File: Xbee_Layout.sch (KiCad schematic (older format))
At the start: 28 parts

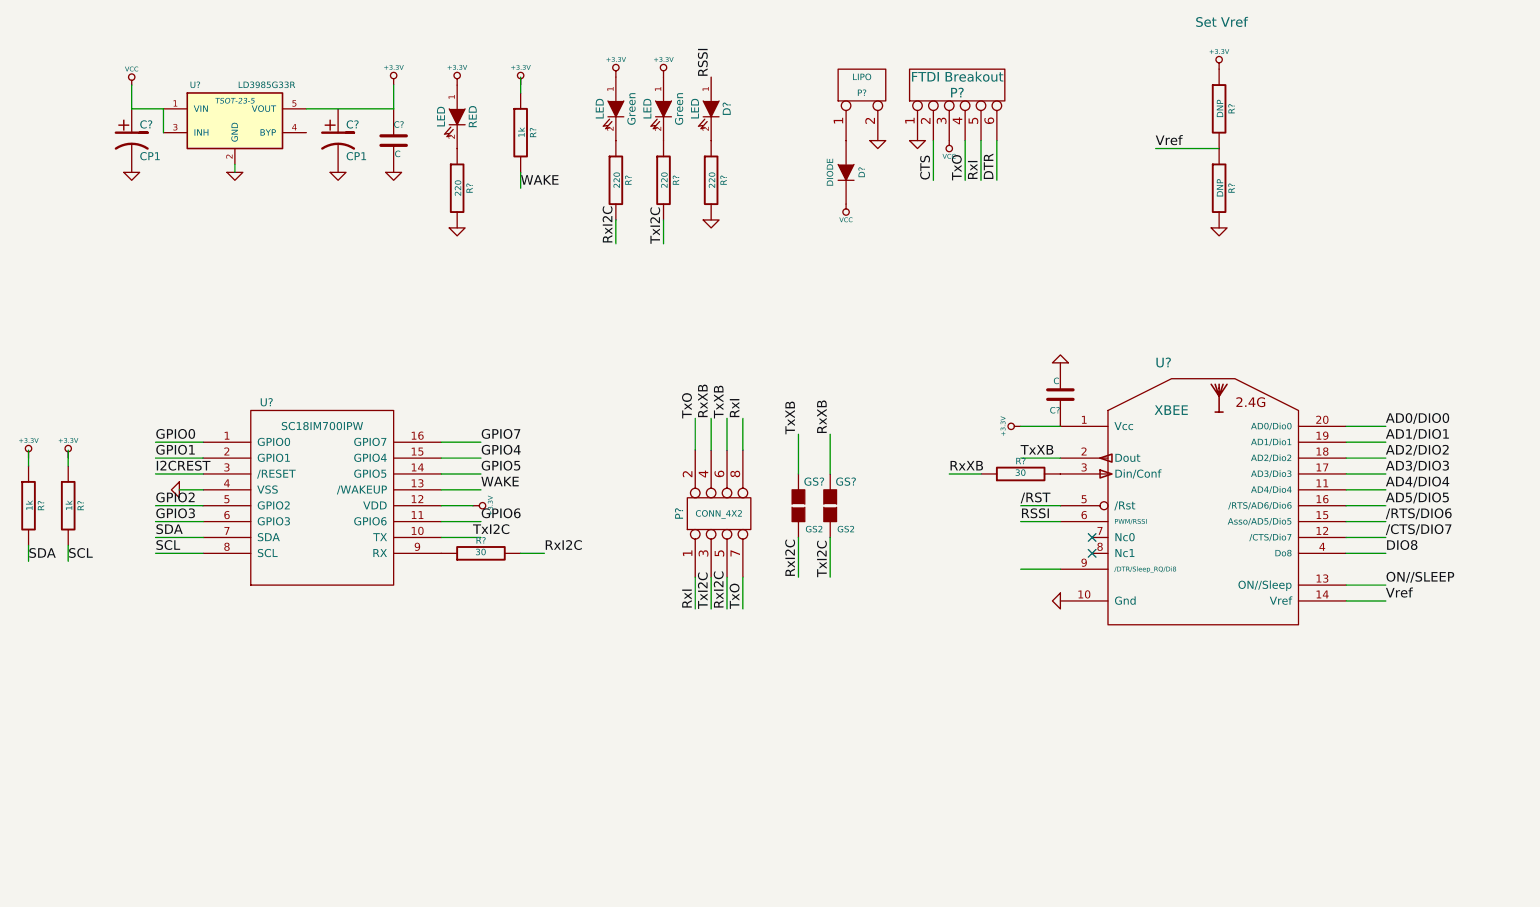
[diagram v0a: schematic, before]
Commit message: Almost finished
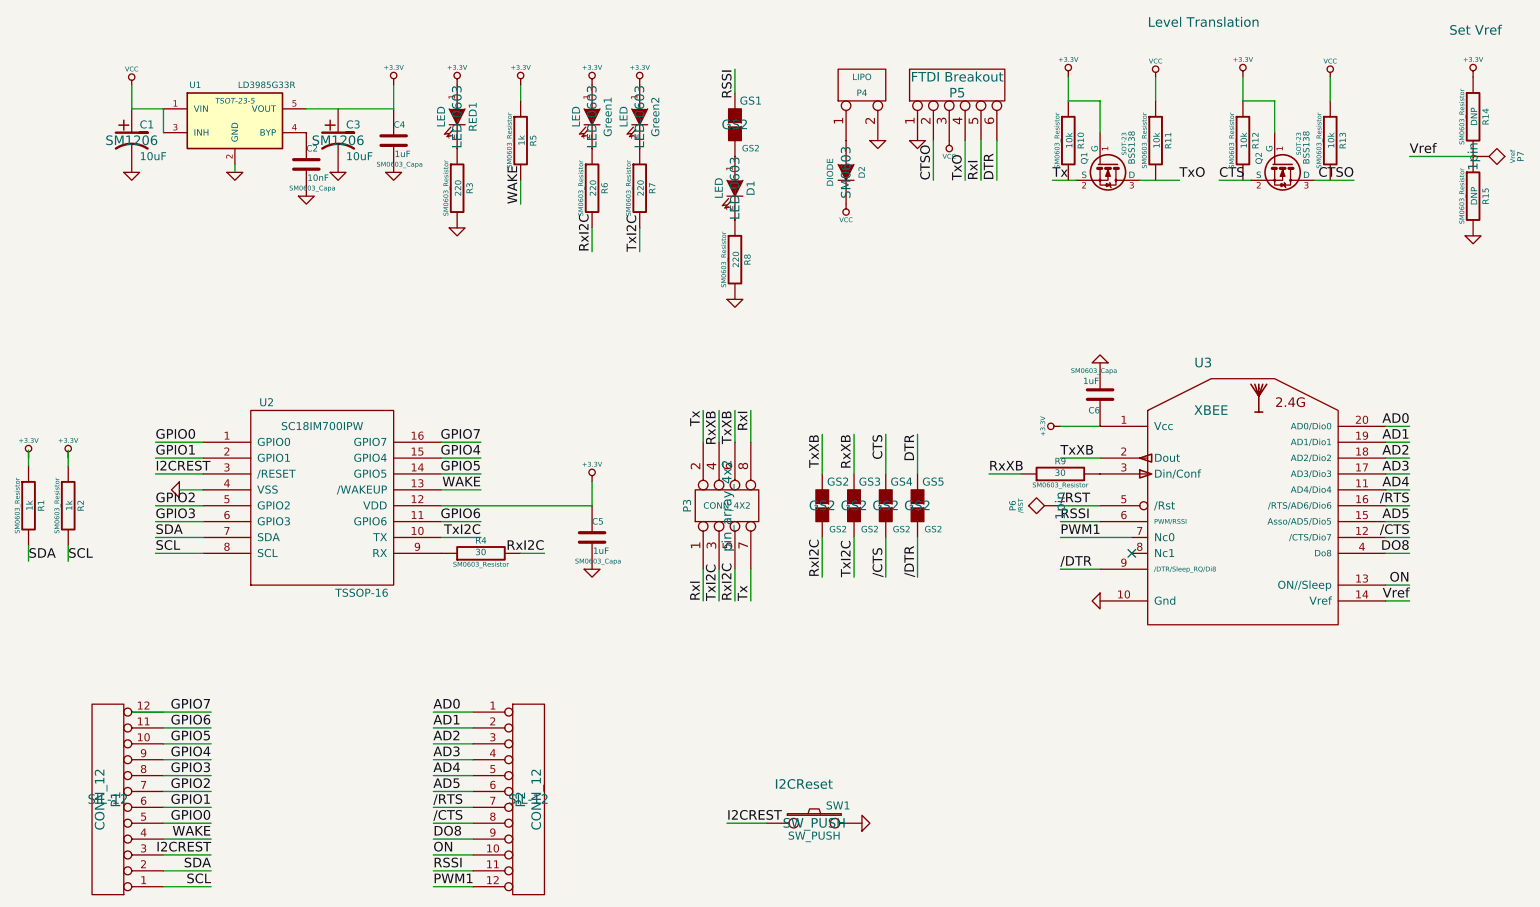
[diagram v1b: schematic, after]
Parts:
- added C2: 10nF, SM0603_Capa, symbol C
- added C5: 1uF, SM0603_Capa, symbol C
- added GS1, GS4, GS5: GS2, GS2, symbol GS2
- added P1, P2: CONN_12, SIL-12, symbol CONN_12
- added P6: /RST, 1pin, symbol TST
- added P7: Vref, 1pin, symbol TST
- added Q1, Q2: BSS138, SOT-23, symbol BSS138
- added R10, R11, R12, R13: 10k, SM0603_Resistor, symbol R
- added SW1: SW_PUSH, SW_PUSH, symbol SW_PUSH
- C1, C3: renamed from C?; value CP1 -> 10uF; footprint ~ -> SM1206
- C4, C6: renamed from C?; value C -> 1uF; footprint ~ -> SM0603_Capa
- D1: renamed from D?; footprint ~ -> LED-0603
- D2: renamed from D?; footprint ~ -> SM0603
- GS2, GS3: renamed from GS?; footprint ~ -> GS2
- Green1, Green2: renamed from Green; footprint ~ -> LED-0603
- P3: renamed from P?; footprint (none) -> pin_array_4x2; Manufacturer (none) -> Molex; Maufacturer Number (none) -> 0901310764
- P4: renamed from P?; Manufacturer (none) -> 4UCON; Manufacturer Number (none) -> Unknown; Vendor (none) -> Sparkfun; Vendor Number (none) -> PRT-08612
- P5: renamed from P?; Manufacturer (none) -> 4UCON; Manufacturer Number (none) -> Unknown; Vendor (none) -> Sparkfun; Vendor Number (none) -> PRT-09015
- R1, R14, R15, R2, R3, R4, R5, R6, R7, R8, R9: renamed from R?; footprint ~ -> SM0603_Resistor
- RED1: renamed from RED; footprint ~ -> LED-0603
- gave numbers to parts that had none: 3
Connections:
- net labels added: /CTS, /DTR, /RTS, AD0, AD1, AD2, AD3, AD4, AD5, CTSO, DO8, ON, PWM1, Tx
- net labels removed: /CTS/DIO7, /RTS/DIO6, AD0/DIO0, AD1/DIO1, AD2/DIO2, AD3/DIO3, AD4/DIO4, AD5/DIO5, DIO8, ON//SLEEP
- wire segments 64 -> 108
- no-connect marks 2 -> 1
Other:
- note added: "I2CReset"
- note added: "Level Translation"
- moved on the sheet: C6, D1, GS2, GS3, Green1, Green2, P3, R14, R15, R5, R6, R7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
